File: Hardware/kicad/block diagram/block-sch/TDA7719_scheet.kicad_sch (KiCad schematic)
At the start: 20 parts, among them J1 AudioJack3, J2 AudioJack3, U5 TDA7719

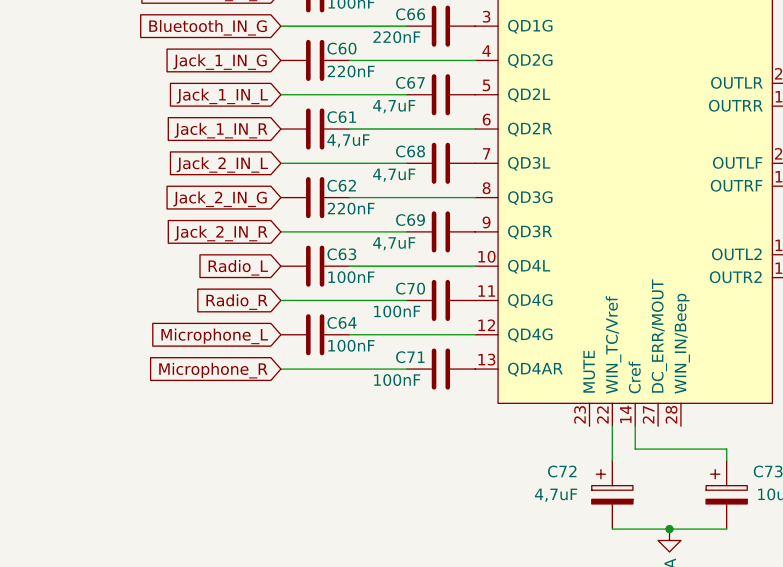
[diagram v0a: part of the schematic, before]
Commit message: new
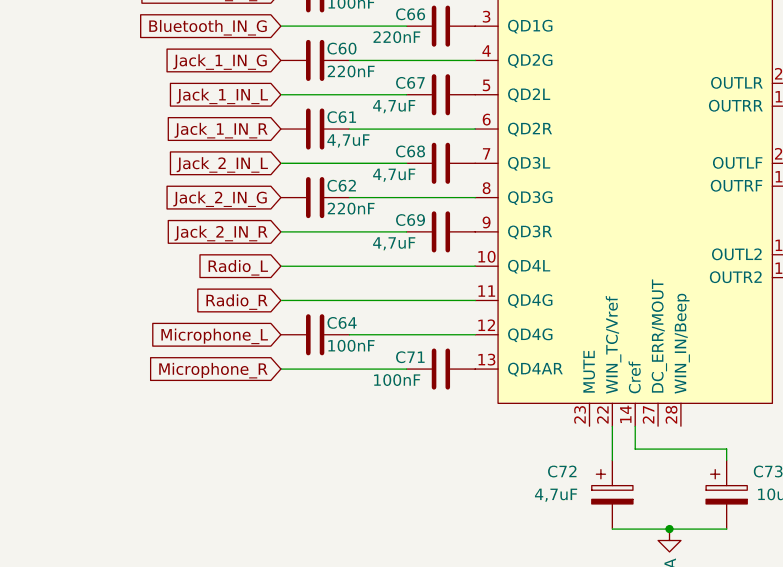
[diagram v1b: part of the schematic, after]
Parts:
- removed C63, C70: 100nF, Capacitor_SMD:C_1206_3216Metric, symbol Device:C
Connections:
- net Radio_L: now also U5.10 (QD4L)
- net Radio_R: now also U5.11 (QD4G)
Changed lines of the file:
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@@
     (stroke (width 0) (type default) (color 0 0 0 0))
   )
-  (wire (pts (xy 66.04 94.996) (xy 80.01 94.996))
+  (wire (pts (xy 58.42 94.996) (xy 80.01 94.996))
     (stroke (width 0) (type default) (color 0 0 0 0))
   )
@@
     (stroke (width 0) (type default) (color 0 0 0 0))
   )
-  (wire (pts (xy 72.39 98.806) (xy 58.42 98.806))
+  (wire (pts (xy 58.42 98.806) (xy 80.01 98.806))
     (stroke (width 0) (type default) (color 0 0 0 0))
   )
@@
       (effects (font (size 1.27 1.27)) hide)
     )
-    (pin "1")
-    (pin "2")
-  )
-  (symbol (lib_id "Device:C") (at 76.2 98.806 270) (unit 1)
-    (in_bom yes) (on_board yes)
-    (property "Reference" "C70" (id 0) (at 71.12 97.536 90)
-      (effects (font (size 1.27 1.27)) (justify left))
-    )
-    (property "Value" "100nF" (id 1) (at 68.58 100.076 90)
-      (effects (font (size 1.27 1.27)) (justify left))
-    )
-    (property "Footprint" "Capacitor_SMD:C_1206_3216Metric" (id 2) (at 72.39 99.7712 0)
-      (effects (font (size 1.27 1.27)) hide)
-    )
-    (property "Datasheet" "~" (id 3) (at 76.2 98.806 0)
-      (effects (font (size 1.27 1.27)) hide)
-    )
-    (pin "1")
-    (pin "2")
-  )
-  (symbol (lib_id "Device:C") (at 62.23 94.996 270) (unit 1)
-    (in_bom yes) (on_board yes)
-    (property "Reference" "C63" (id 0) (at 63.5 93.726 90)
-      (effects (font (size 1.27 1.27)) (justify left))
-    )
-    (property "Value" "100nF" (id 1) (at 63.5 96.266 90)
-      (effects (font (size 1.27 1.27)) (justify left))
-    )
-    (property "Footprint" "Capacitor_SMD:C_1206_3216Metric" (id 2) (at 58.42 95.9612 0)
-      (effects (font (size 1.27 1.27)) hide)
-    )
-    (property "Datasheet" "~" (id 3) (at 62.23 94.996 0)
-      (effects (font (size 1.27 1.27)) hide)
-    )

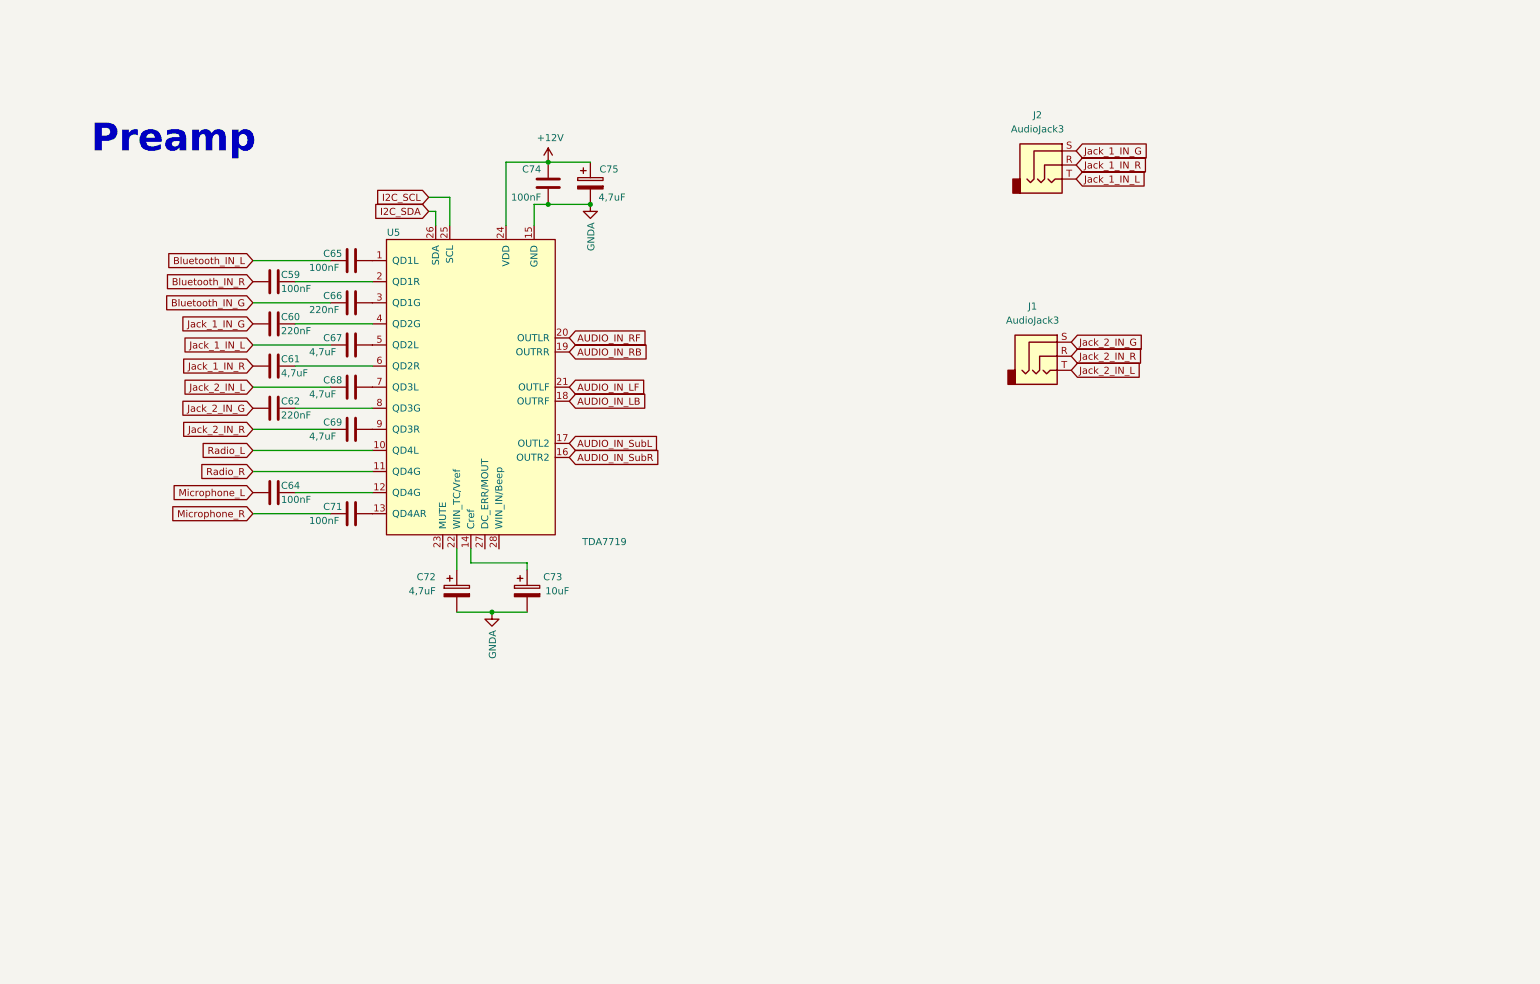
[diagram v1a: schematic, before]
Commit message: new
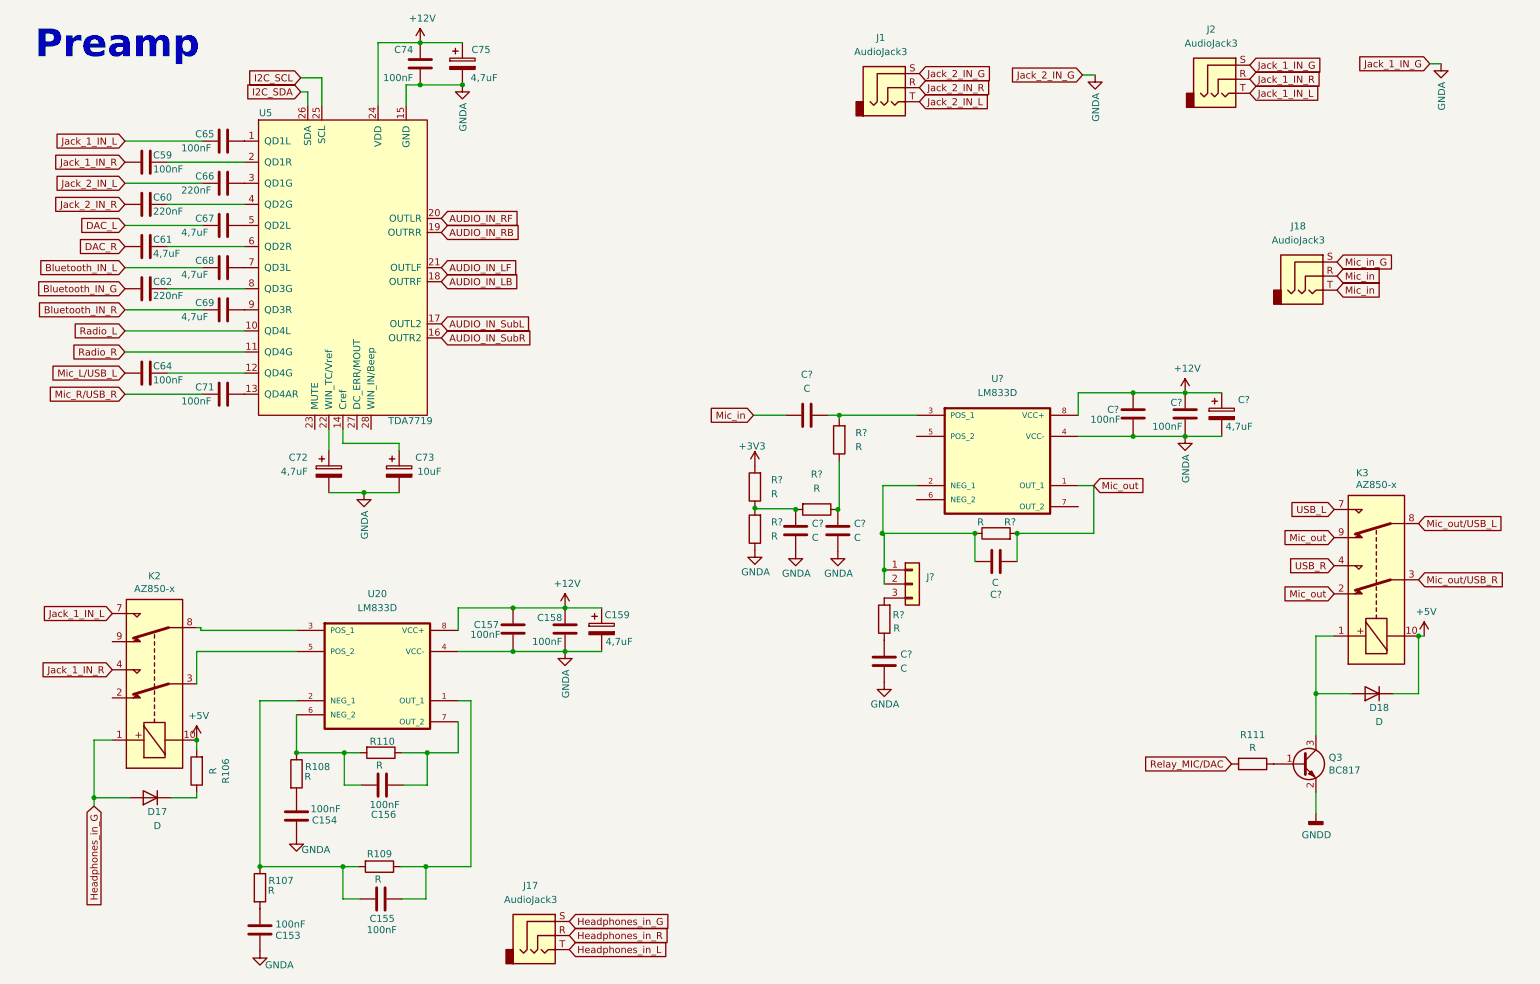
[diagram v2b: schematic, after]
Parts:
- added C153, C154, C155, C156, C157, C158, C? (x2): 100nF, Capacitor_SMD:C_1206_3216Metric, symbol Device:C
- added C159, C?: 4,7uF, Capacitor_THT:CP_Radial_D6.3mm_P2.50mm, symbol Device:CP
- added C? (x5): C, Capacitor_SMD:C_0805_2012Metric, symbol Device:C
- added D17, D18: D, Diode_THT:D_DO-35_SOD27_P7.62mm_Horizontal, symbol Device:D
- added J17, J18: AudioJack3, Connector_Audio:Jack_3.5mm_CUI_SJ1-3533NG_Horizontal, symbol Connector:AudioJack3
- added J?: Conn_01x03, Connector_PinHeader_1.27mm:PinHeader_1x03_P1.27mm_Vertical, symbol Connector_Generic:Conn_01x03
- added K2, K3: AZ850-x, Relay_THT:Relay_DPDT_Fujitsu_FTR-F1C, symbol Relay:AZ850-x
- added Q3: BC817, Package_TO_SOT_SMD:SOT-23, symbol Electronic_stethoscope-cache:Transistor_BJT_BC817
- added R106, R107, R108, R109, R110, R111: R, Resistor_SMD:R_1206_3216Metric, symbol Device:R
- added R? (x6): R, Resistor_SMD:R_0805_2012Metric, symbol Device:R
- added U20, U?: LM833D, SOIC127P599X175-8N, symbol amplituner_lib_sym:LM833D
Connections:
- net +12V: now also C157.2, C158.2, C159.1, C?.1, C?.2, C?.2, U20.8 (VCC+), U?.8 (VCC+)
- net Bluetooth_IN_G: now also C62.2; no longer C66.2
- net Bluetooth_IN_L: now also C68.2; no longer C65.2
- net Bluetooth_IN_R: now also C69.2; no longer C59.2
- net GNDA: now also J1.S, J2.S, C153.2, C154.2, C157.1, C158.1, C159.2, C?.1, C?.1, C?.1, C?.1, C?.1, C?.2, R?.1, U20.4 (VCC-), U?.4 (VCC-)
- net Jack_1_IN_L: now also C65.2, K2.7; no longer C67.2
- net Jack_1_IN_R: now also C59.2, K2.4; no longer C61.2
- net Jack_2_IN_L: now also C66.2; no longer C68.2
- net Jack_2_IN_R: now also C60.2; no longer C69.2
- removed net Jack_1_IN_G: C60.2, J2.S
- removed net Jack_2_IN_G: C62.2, J1.S
- net Microphone_L renamed Mic_L/USB_L
- net Microphone_R renamed Mic_R/USB_R
- new net: C?.2, R?.1, R?.2, R?.2
- new net: K2.3, U20.5 (POS_2)
- new net: K2.8, U20.3 (POS_1)
- new net: J?.1 (Pin_1), J?.2 (Pin_2), U?.2 (NEG_1)
- new net: C?.1, R?.2, U?.3 (POS_1)
- new net: D18.2 (A), K3.1, Q3.3 (C)
- new net: C154.1, R108.2
- new net: C?.2, R?.1
- new net: C?.2, R?.1, R?.1
- new net: C?.1, R?.1
- new net: Q3.1 (B), R111.1
- new net: D17.1 (K), R106.1
- new net: J?.3 (Pin_3), R?.2
- new net: C156.1, R110.1, U20.7 (OUT_2)
- new net: C156.2, R108.1, R110.2, U20.6 (NEG_2)
- new net: C153.1, R107.2
- new net: C155.1, R109.1, U20.1 (OUT_1)
- new net: C155.2, R107.1, R109.2, U20.2 (NEG_1)
- new net +3V3: R?.2
- new net +5V: D18.1 (K), K2.10, K3.10, R106.2
- new net DAC_L: C67.2
- new net DAC_R: C61.2
- new net GNDD: Q3.2 (E)
- new net Headphones_in_G: D17.2 (A), J17.S, K2.1
- new net Headphones_in_L: J17.T
- new net Headphones_in_R: J17.R
- new net Mic_in: C?.2, J18.R, J18.T
- new net Mic_in_G: J18.S
- new net Mic_out: C?.2, K3.2, K3.9, R?.2, U?.1 (OUT_1)
- new net Mic_out/USB_L: K3.8
- new net Mic_out/USB_R: K3.3
- new net Relay_MIC/DAC: R111.2
- new net USB_L: K3.7
- new net USB_R: K3.4
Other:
- moved on the sheet: C59, C60, C61, C62, C64, C65, C66, C67, C68, C69, C71, C72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

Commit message: new
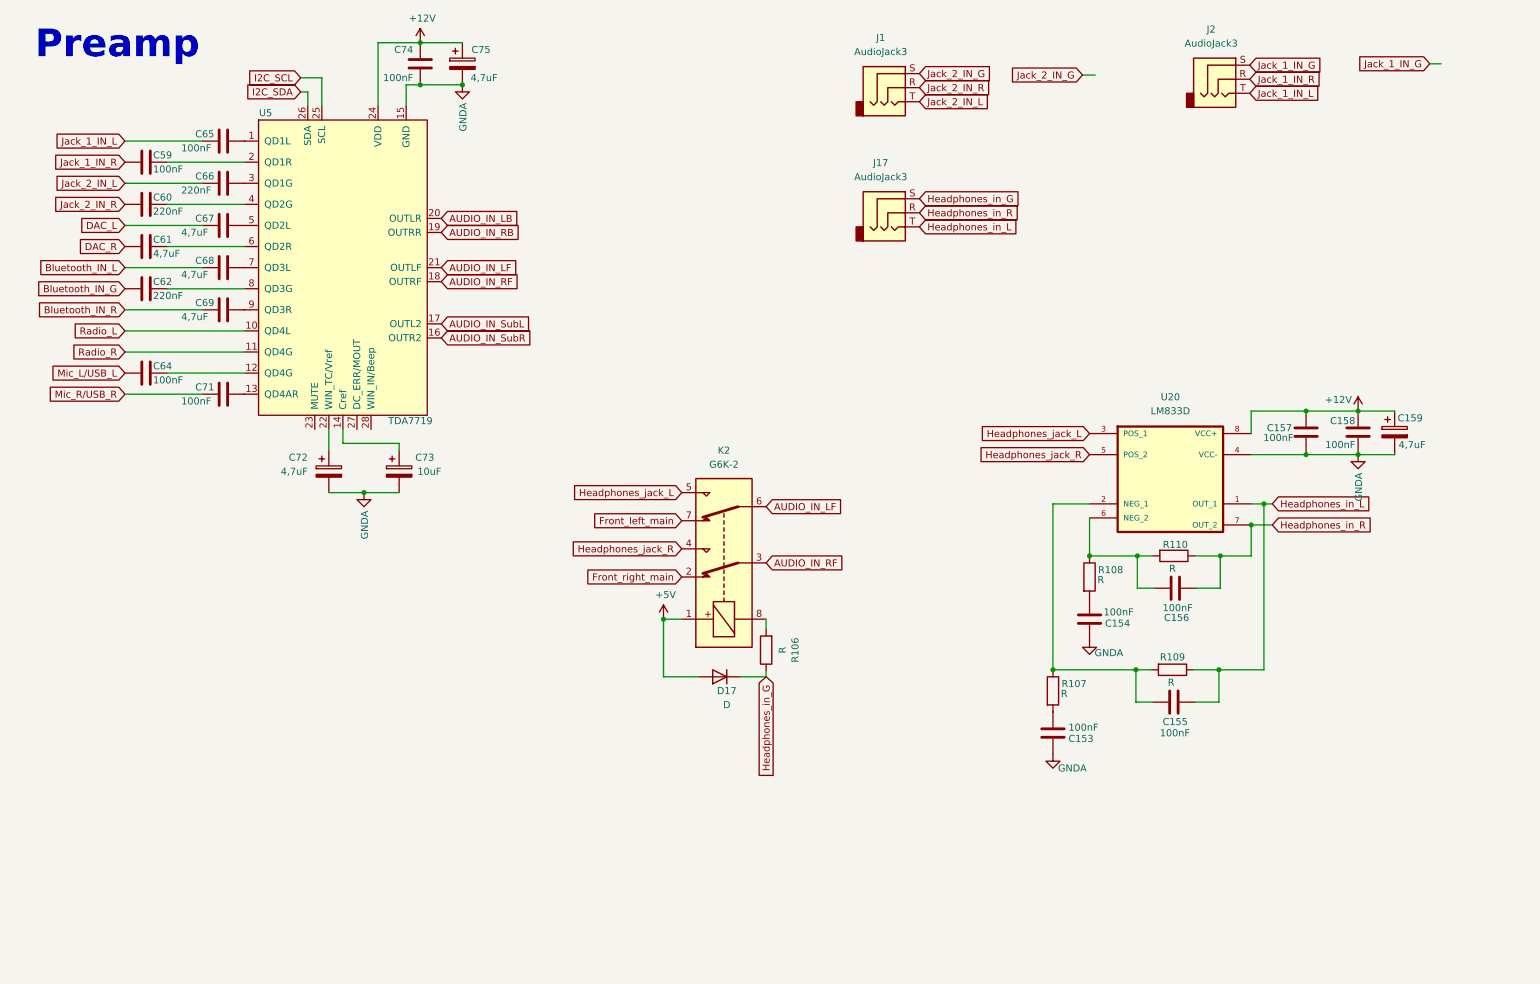
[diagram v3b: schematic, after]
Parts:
- removed C?: 4,7uF, Capacitor_THT:CP_Radial_D6.3mm_P2.50mm, symbol Device:CP
- removed C? (x5): C, Capacitor_SMD:C_0805_2012Metric, symbol Device:C
- removed C? (x2): 100nF, Capacitor_SMD:C_1206_3216Metric, symbol Device:C
- removed D18: D, Diode_THT:D_DO-35_SOD27_P7.62mm_Horizontal, symbol Device:D
- removed J18: AudioJack3, Connector_Audio:Jack_3.5mm_CUI_SJ1-3533NG_Horizontal, symbol Connector:AudioJack3
- removed J?: Conn_01x03, Connector_PinHeader_1.27mm:PinHeader_1x03_P1.27mm_Vertical, symbol Connector_Generic:Conn_01x03
- removed K2, K3: AZ850-x, Relay_THT:Relay_DPDT_Fujitsu_FTR-F1C, symbol Relay:AZ850-x
- removed Q3: BC817, Package_TO_SOT_SMD:SOT-23, symbol Electronic_stethoscope-cache:Transistor_BJT_BC817
- removed R111: R, Resistor_SMD:R_1206_3216Metric, symbol Device:R
- removed R? (x6): R, Resistor_SMD:R_0805_2012Metric, symbol Device:R
- removed U?: LM833D, SOIC127P599X175-8N, symbol amplituner_lib_sym:LM833D
- added K2: G6K-2, Relay_SMD:Relay_DPDT_Omron_G6K-2F-Y, symbol Relay:G6K-2
- U20: footprint SOIC127P599X175-8N -> amplituner_lib:LMV358
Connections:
- net +5V: now also D17.2 (A), K2.1; no longer R106.2
- net AUDIO_IN_LB: now also U5.20 (OUTLR); no longer U5.18 (OUTRF)
- net AUDIO_IN_LF: now also K2.6
- net AUDIO_IN_RF: now also U5.18 (OUTRF), K2.3; no longer U5.20 (OUTLR)
- net GNDA: no longer J1.S, J2.S
- net Headphones_in_G: now also D17.1 (K), R106.1; no longer D17.2 (A)
- net Headphones_in_L: now also C155.1, R109.1, U20.1 (OUT_1)
- net Headphones_in_R: now also C156.1, R110.1, U20.7 (OUT_2)
- net Headphones_jack_R: now reaches U20.5 (POS_2)
- net Headphones_jack_R: now also K2.4
- net Headphones_jack_L: now reaches U20.3 (POS_1)
- net Headphones_jack_L: now also K2.5
- new net: K2.8, R106.2
- new net Front_left_main: K2.7
- new net Front_right_main: K2.2
- new net Jack_1_IN_G: J2.S
- new net Jack_2_IN_G: J1.S
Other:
- moved on the sheet: C153, C154, C155, C156, C157, C158, C159, D17, J17, R106, R107, R108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

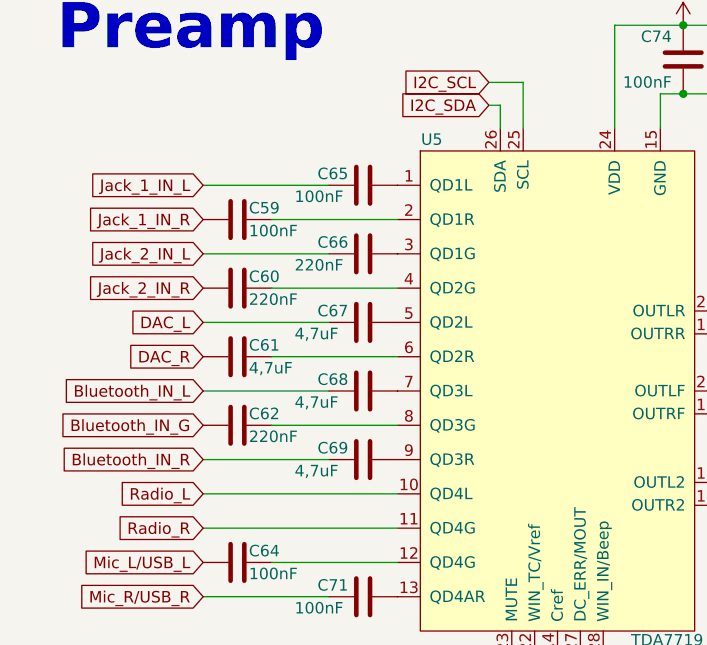
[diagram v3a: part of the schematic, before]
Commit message: new
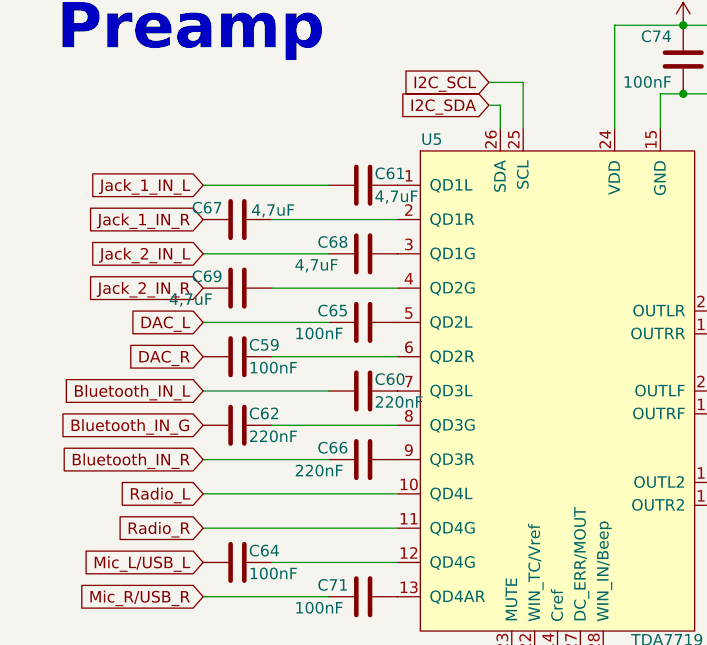
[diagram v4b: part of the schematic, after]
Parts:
- R106: footprint Resistor_SMD:R_1206_3216Metric -> Resistor_SMD:R_0805_2012Metric
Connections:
- net Bluetooth_IN_L: now also C60.2; no longer C68.2
- net Bluetooth_IN_R: now also C66.2; no longer C69.2
- net DAC_L: now also C65.2; no longer C67.2
- net DAC_R: now also C59.2; no longer C61.2
- net Jack_1_IN_L: now also C61.2; no longer C65.2
- net Jack_1_IN_R: now also C67.2; no longer C59.2
- net Jack_2_IN_L: now also C68.2; no longer C66.2
- net Jack_2_IN_R: now also C69.2; no longer C60.2
- net at U5.1 (QD1L): now also C61.1; no longer C65.1
- net at U5.2 (QD1R): now also C67.1; no longer C59.1
- net at U5.3 (QD1G): now also C68.1; no longer C66.1
- net at U5.4 (QD2G): now also C69.1; no longer C60.1
- net at U5.5 (QD2L): now also C65.1; no longer C67.1
- net at U5.6 (QD2R): now also C59.1; no longer C61.1
- net at U5.7 (QD3L): now also C60.1; no longer C68.1
- net at U5.9 (QD3R): now also C66.1; no longer C69.1
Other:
- moved on the sheet: C59, C60, C61, C65, C66, C67, C68, C69
